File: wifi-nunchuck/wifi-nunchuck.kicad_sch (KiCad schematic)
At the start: 22 parts, among them J2 USB_B_Micro, Q1 BSS138, Q2 BSS138, U1 ESP32-WROOM-32, U2 AMS1117-3.3, U3 CH340C

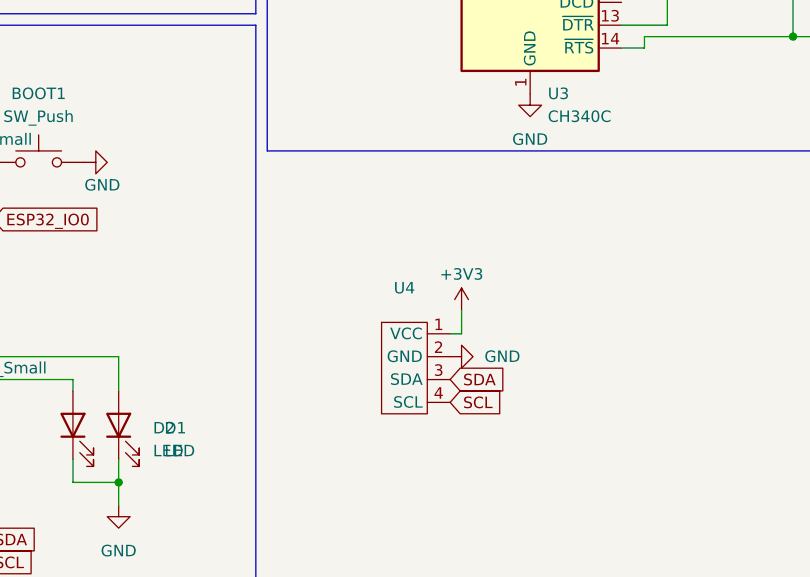
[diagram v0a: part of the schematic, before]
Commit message: add views
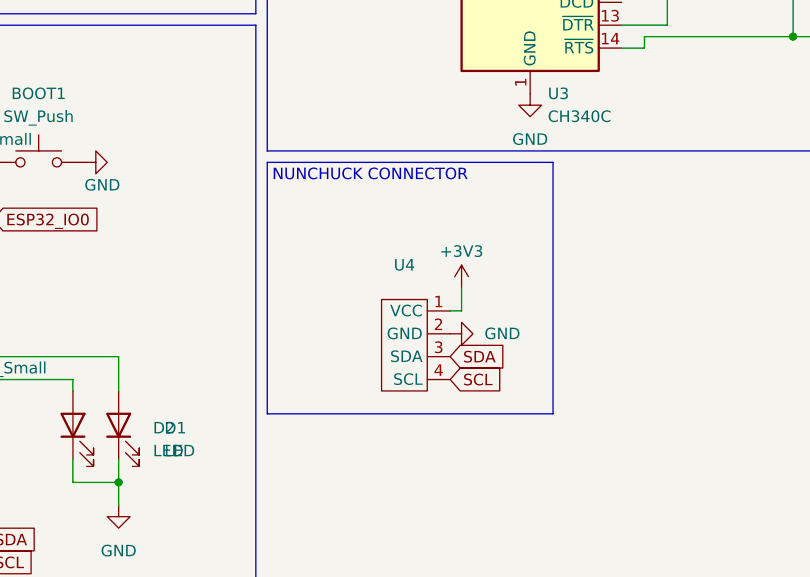
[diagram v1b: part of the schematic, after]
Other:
- note added: "NUNCHUCK CONNECTOR"
- moved on the sheet: U4
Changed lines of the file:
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@@
 	(wire
 		(pts
-			(xy 134.62 83.82) (xy 134.62 81.28)
-		)
-		(stroke
-			(width 0)
-			(type default)
-		)
-	)
-	(wire
-		(pts
-			(xy 133.35 83.82) (xy 134.62 83.82)
+			(xy 134.62 81.28) (xy 134.62 78.74)
+		)
+		(stroke
+			(width 0)
+			(type default)
+		)
+	)
+	(wire
+		(pts
+			(xy 133.35 81.28) (xy 134.62 81.28)
 		)
 		(stroke
@@
 			(width 0)
 			(type default)
+		)
+	)
+	(rectangle
+		(start 113.03 64.77)
+		(end 144.78 92.71)
+		(stroke
+			(width 0)
+			(type default)
+		)
+		(fill
+			(type none)
 		)
 	)
@@
 		)
 	)
+	(text "NUNCHUCK CONNECTOR"
+		(exclude_from_sim no)
+		(at 124.46 66.294 0)
+		(effects
+			(font
+				(size 1.27 1.27)
+			)
+		)
+	)
 	(text "REGULATOR"
 		(exclude_from_sim no)
@@
 	(global_label "SDA"
 		(shape input)
-		(at 133.35 88.9 0)
+		(at 133.35 86.36 0)
 		(fields_autoplaced yes)
 		(effects
@@
 		)
 		(property "Intersheetrefs" "${INTERSHEET_REFS}"
-			(at 139.9033 88.9 0)
+			(at 139.9033 86.36 0)
 			(effects
 				(font
@@
 	(global_label "SCL"
 		(shape input)
-		(at 133.35 91.44 0)
+		(at 133.35 88.9 0)
 		(fields_autoplaced yes)
 		(effects
@@
 		)
 		(property "Intersheetrefs" "${INTERSHEET_REFS}"
-			(at 139.8428 91.44 0)
+			(at 139.8428 88.9 0)
 			(effects
 				(font
@@
 	(symbol
 		(lib_id "Nunchuck:Nunchuck")
-		(at 128.27 82.55 0)
+		(at 128.27 80.01 0)
 		(unit 1)
 		(exclude_from_sim no)
@@
 		(fields_autoplaced yes)
 		(property "Reference" "U4"
+			(at 128.27 76.2 0)
+			(effects
+				(font
+					(size 1.27 1.27)
+				)
+			)
+		)
+		(property "Value" "~"
 			(at 128.27 78.74 0)
 			(effects
@@
 			)
 		)
-		(property "Value" "~"
-			(at 128.27 81.28 0)
-			(effects
-				(font
-					(size 1.27 1.27)
-				)
-			)
-		)
 		(property "Footprint" "wii:nunchuck"
-			(at 128.27 82.55 0)
+			(at 128.27 80.01 0)
 			(effects
 				(font
@@
 		)
 		(property "Datasheet" ""
-			(at 128.27 82.55 0)
-			(effects
-				(font
-					(size 1.27 1.27)
-				)
-				(hide yes)
-			)
-		)
-		(property "Description" ""
-			(at 128.27 82.55 0)
+			(at 128.27 80.01 0)
+			(effects
+				(font
+					(size 1.27 1.27)
+				)
+				(hide yes)
+			)
+		)
+		(property "Description" ""
+			(at 128.27 80.01 0)
 			(effects
 				(font
@@
 	(symbol
 		(lib_id "power:+3V3")
-		(at 134.62 81.28 0)
+		(at 134.62 78.74 0)
 		(unit 1)
 		(exclude_from_sim no)
@@
 		(dnp no)
 		(property "Reference" "#PWR019"
-			(at 134.62 85.09 0)
+			(at 134.62 82.55 0)
 			(effects
 				(font
@@
 		)
 		(property "Value" "+3V3"
-			(at 134.62 77.216 0)
+			(at 134.62 74.676 0)
 			(effects
 				(font
@@
 		)
 		(property "Footprint" ""
-			(at 134.62 81.28 0)
+			(at 134.62 78.74 0)
 			(effects
 				(font
@@
 		)
 		(property "Datasheet" ""
-			(at 134.62 81.28 0)
-			(effects
-				(font
-					(size 1.27 1.27)
-				)
-				(hide yes)
-			)
-		)
-		(property "Description" ""
-			(at 134.62 81.28 0)
+			(at 134.62 78.74 0)
+			(effects
+				(font
+					(size 1.27 1.27)
+				)
+				(hide yes)
+			)
+		)
+		(property "Description" ""
+			(at 134.62 78.74 0)
 			(effects
 				(font
@@
 	(symbol
 		(lib_id "power:GND")
-		(at 133.35 86.36 90)
+		(at 133.35 83.82 90)
 		(unit 1)
 		(exclude_from_sim no)
@@
 		(fields_autoplaced yes)
 		(property "Reference" "#PWR018"
-			(at 139.7 86.36 0)
+			(at 139.7 83.82 0)
 			(effects
 				(font
@@
 		)
 		(property "Value" "GND"
-			(at 137.16 86.3599 90)
+			(at 137.16 83.8199 90)
 			(effects
 				(font
@@
 		)
 		(property "Footprint" ""
-			(at 133.35 86.36 0)
+			(at 133.35 83.82 0)
 			(effects
 				(font
@@
 		)
 		(property "Datasheet" ""
-			(at 133.35 86.36 0)
-			(effects
-				(font
-					(size 1.27 1.27)
-				)
-				(hide yes)
-			)
-		)
-		(property "Description" ""
-			(at 133.35 86.36 0)
-			(effects
-				(font
+			(at 133.35 83.82 0)
+			(effects
+				(font
+					(size 1.27 1.27)
+				)
+				(hide yes)
+			)
+		)
+		(property "Description" ""
+			(at 133.35 83.82 0)
+			(effects
+				(font
